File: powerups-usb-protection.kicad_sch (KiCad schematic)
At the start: 2 parts, among them P1 USB_C_Plug_USB2.0, P2 USB_C_Plug_USB2.0

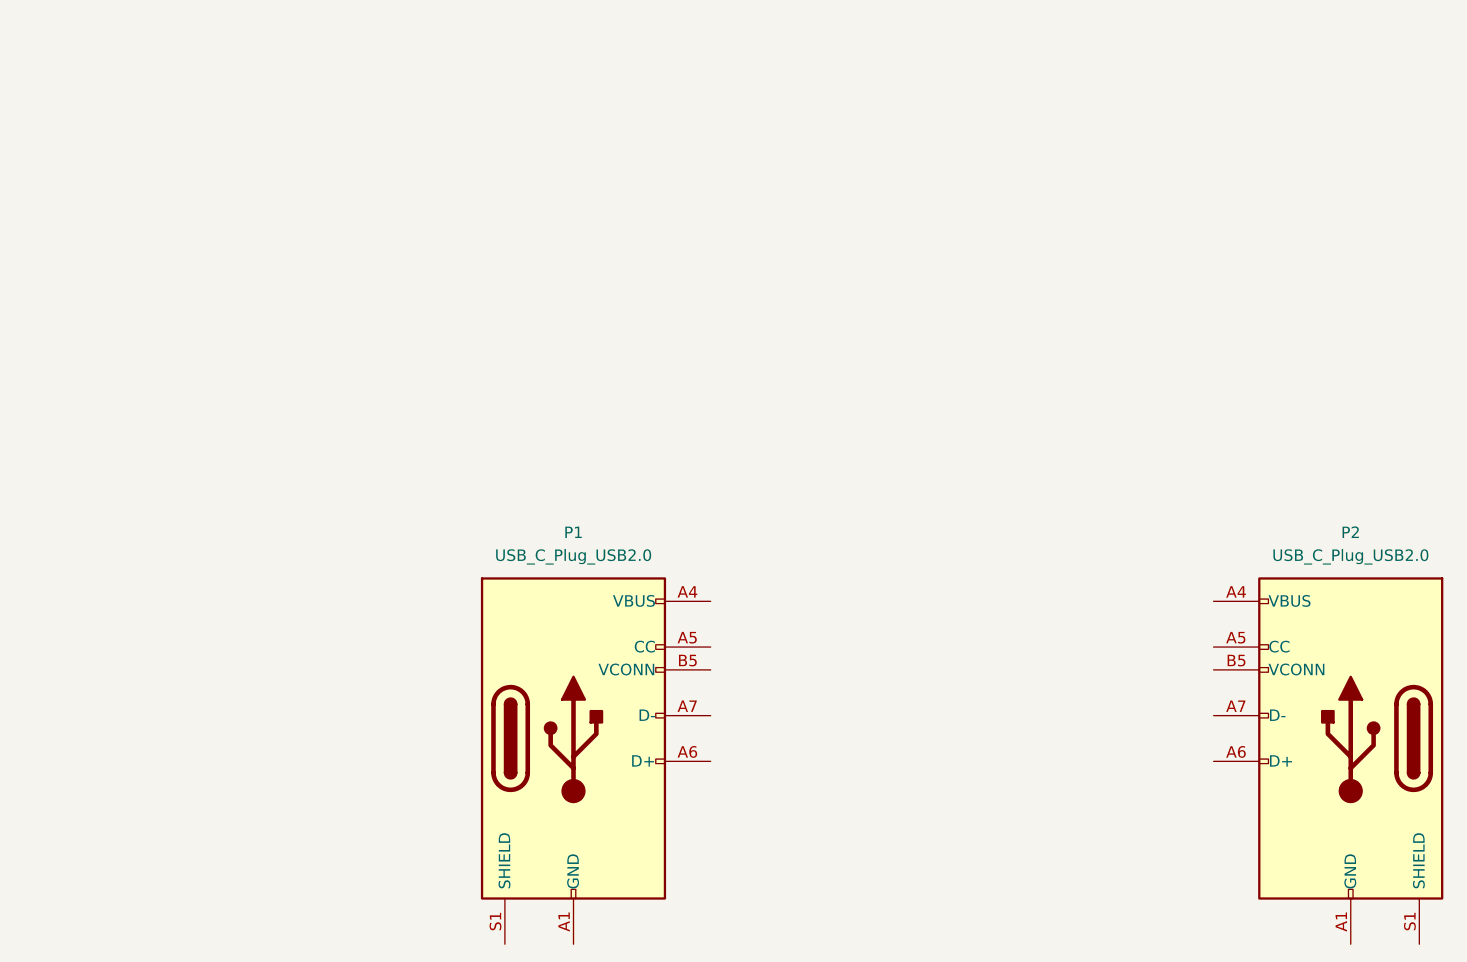
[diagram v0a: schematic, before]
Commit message: First schematic and layout
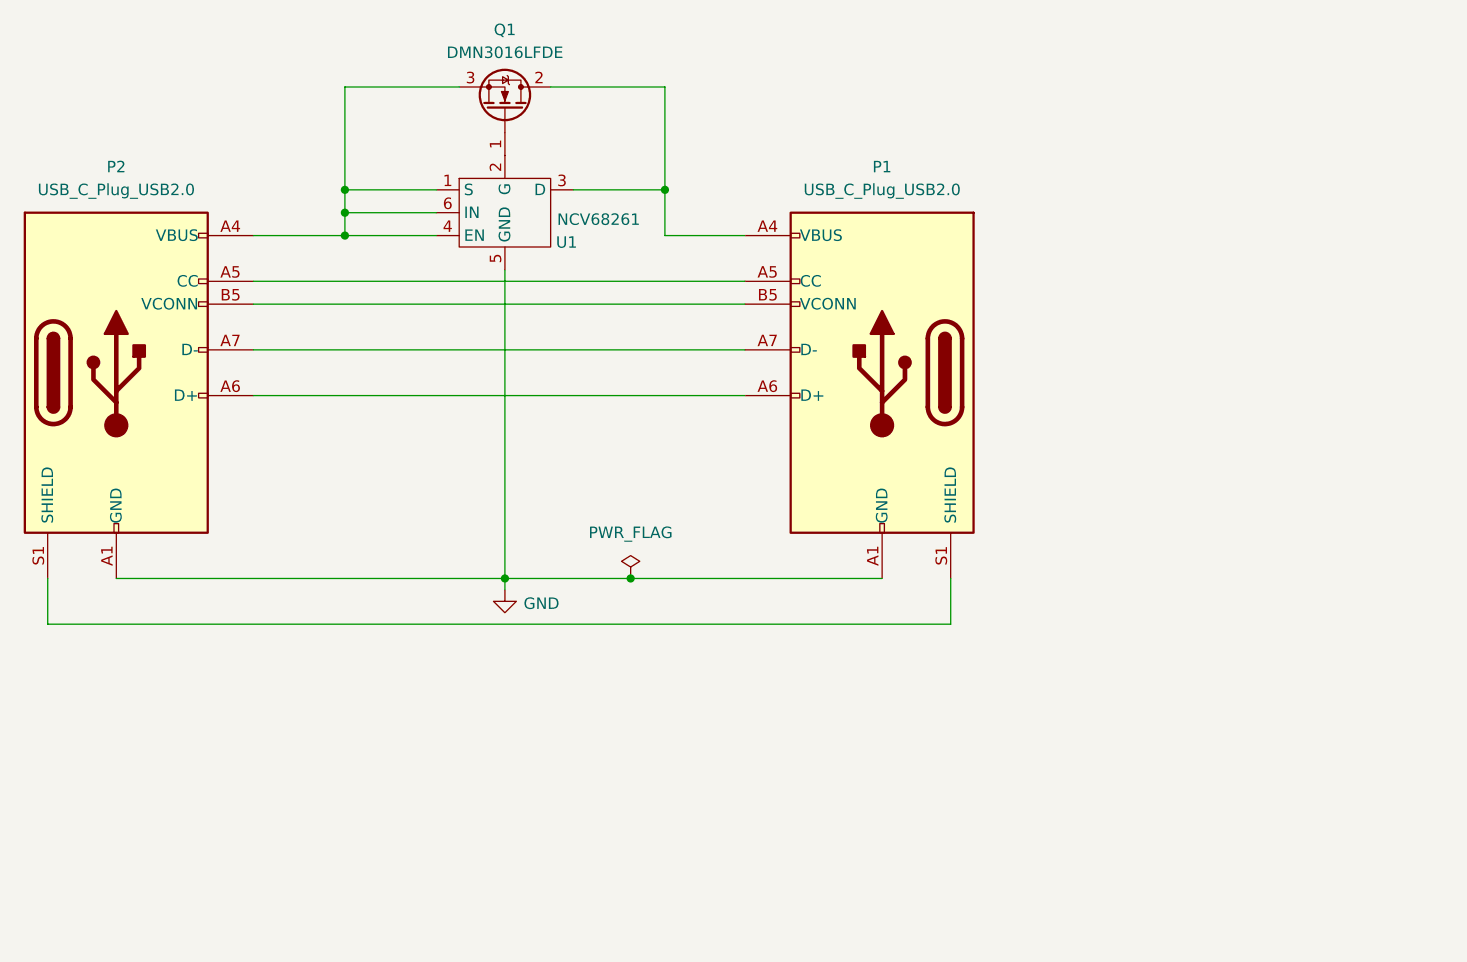
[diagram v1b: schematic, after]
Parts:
- added Q1: DMN3016LFDE, PowerFeather_KiCAD_Lib:DMN3016LFDE, symbol Device:Q_NMOS_GDS
- added U1: NCV68261, PowerFeather_KiCAD_Lib:DFN-6_2x2mm_P0.65mm_EP1x1.6mm, symbol PowerFeather_KiCAD_Lib:NCV68261
- P1, P2: footprint (none) -> Connector_USB:USB_C_Receptacle_HRO_TYPE-C-31-M-12
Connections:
- net GND: now reaches P2.A1 (GND), P2.A12 (GND), P2.B1 (GND), P2.B12 (GND)
- net GND: now also P1.A1 (GND), P1.A12 (GND), P1.B1 (GND), P1.B12 (GND), U1.5 (GND)
- net at P2.A4 (VBUS), P2.A9 (VBUS), P2.B4 (VBUS)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: now also Q1.3 (S), U1.1 (S), U1.4 (EN), U1.6 (IN)
- net at P2.A5 (CC): now also P1.A5 (CC)
- net at P2.A6 (D+): now also P1.A6 (D+)
- net at P2.A7 (D-): now also P1.A7 (D-)
- net at P2.B5 (VCONN): now also P1.B5 (VCONN)
- net at P2.S1 (SHIELD): now also P1.S1 (SHIELD)
- net at P1.A4 (VBUS), P1.A9 (VBUS), P1.B4 (VBUS)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: now also Q1.2 (D), U1.3 (D)
- new net: Q1.1 (G), U1.2 (G)
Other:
- moved on the sheet: P1, P2
